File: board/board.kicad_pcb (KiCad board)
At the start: 2 copper layers, 21 x 13 mm, 1 part

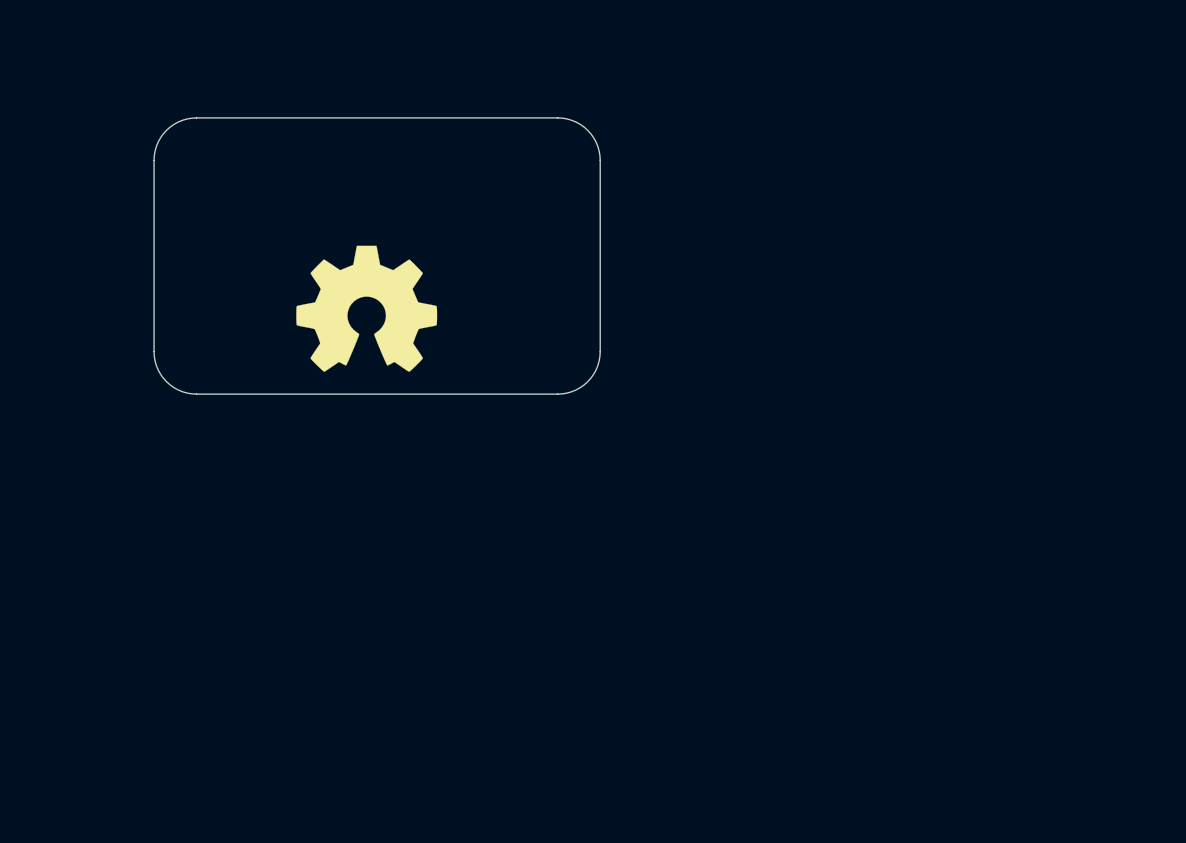
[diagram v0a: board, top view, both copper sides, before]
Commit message: initial
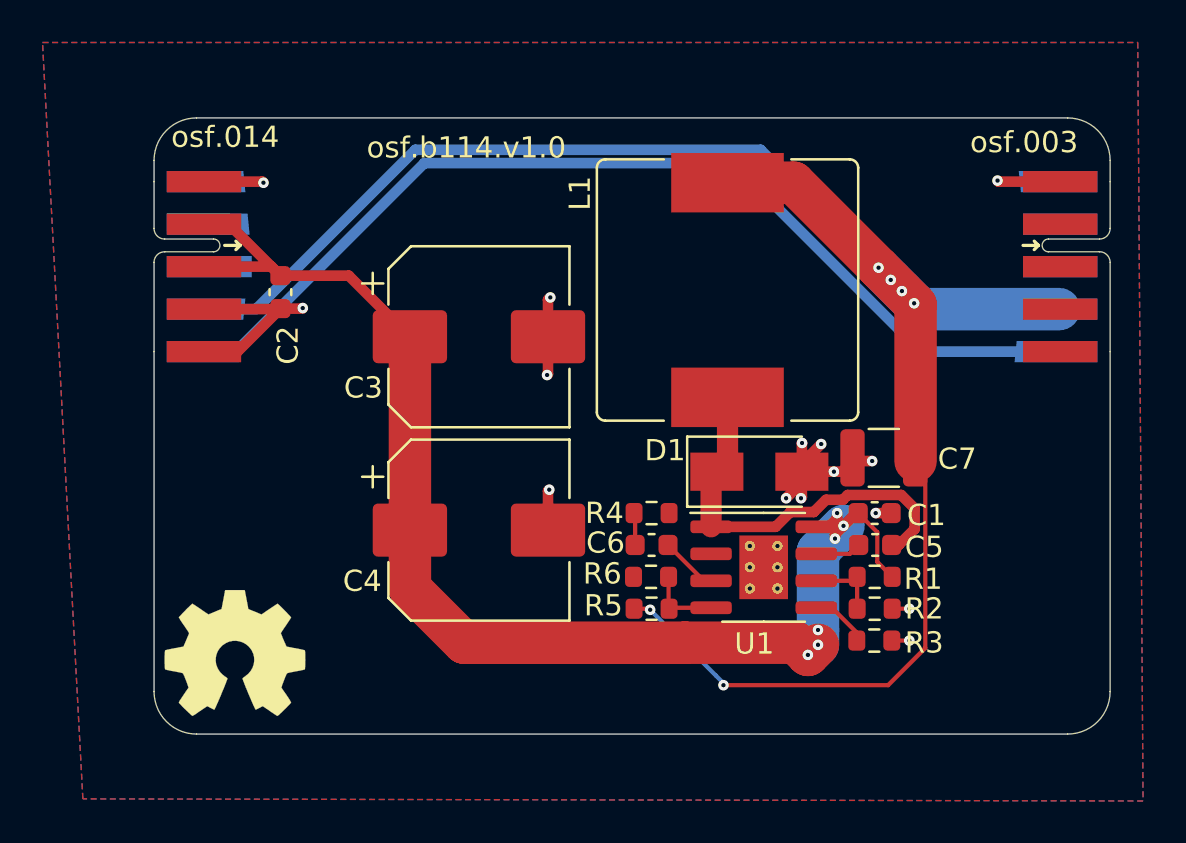
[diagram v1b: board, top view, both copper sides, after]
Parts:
- added C1: 100nF, Capacitor_SMD:C_0603_1608Metric, F.Cu at (173.9, 108.6)
- added C2: 100nF, Capacitor_SMD:C_0603_1608Metric, F.Cu at (145.9, 98.2)
- added C3: 22uF, Capacitor_SMD:CP_Elec_8x10, F.Cu at (155.3, 100.3)
- added C4: 22uF, Capacitor_SMD:CP_Elec_8x10, F.Cu at (155.3, 109.4)
- added C5: 100nF, Capacitor_SMD:C_0603_1608Metric, F.Cu at (173.9, 110.1)
- added C6: 6.8nF, Capacitor_SMD:C_0603_1608Metric, F.Cu at (163.4, 110.1)
- added C7: 100uF, Capacitor_SMD:C_1210_3225Metric, F.Cu at (174.3, 106.0)
- added D1: NRVTSA4100ET3G, Diode_SMD:D_SMA, F.Cu at (168.5, 106.7)
- added J1: 014_PoE_controlled, on_edge:on_edge_2x05_device, F.Cu at (140.0, 97.0)
- added J2: 003_power, on_edge:on_edge_2x05_host, F.Cu at (185.0, 97.0)
- added L1: 33uH, Inductor_SMD:L_Bourns_SRR1210A, F.Cu at (167.0, 98.1)
- added R1: 510k, Resistor_SMD:R_0603_1608Metric, F.Cu at (173.9, 111.6)
- added R2: 100k, Resistor_SMD:R_0603_1608Metric, F.Cu at (173.9, 113.1)
- added R3: 47k, Resistor_SMD:R_0603_1608Metric, F.Cu at (173.9, 114.6)
- added R4: 10k, Resistor_SMD:R_0603_1608Metric, F.Cu at (163.4, 108.6)
- added R5: 2.3k, Resistor_SMD:R_0603_1608Metric, F.Cu at (163.4, 113.1)
- added R6: 1k, Resistor_SMD:R_0603_1608Metric, F.Cu at (163.4, 111.6)
- added U1: BD9G341AEFJ-E2, Package_SO:SOIC-8-1EP_3.9x4.9mm_P1.27mm_EP2.29x3mm_ThermalVias, F.Cu at (168.7, 111.2)
- moved LOGO1 17.3 mm to (143.8, 115.2)
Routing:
- net /step-down/out: track 0.00 -> 90.0 mm, vias 0 -> 6
- net /step-down/in: track 0.00 -> 62.3 mm, vias 0 -> 6
- net Net-(J1-Pad10): track 0.00 -> 47.6 mm
- net GND: track 0.00 -> 32.3 mm, vias 0 -> 15
- net Net-(C5-Pad1): track 0.00 -> 19.2 mm
- net Net-(R5-Pad2): track 0.00 -> 3.50 mm
- net Net-(R1-Pad2): track 0.00 -> 3.50 mm
- net Net-(R3-Pad1): track 0.00 -> 2.77 mm
- net Net-(C6-Pad1): track 0.00 -> 2.72 mm
- net Net-(C5-Pad2): track 0.00 -> 2.17 mm
- net Net-(C6-Pad2): track 0.00 -> 1.52 mm
- added copper zone on B.Cu, net GND
- added copper zone on F.Cu, net GND
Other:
- board size 21 x 13 mm -> 45 x 29 mm
- board text added: "osf.003"
- board text added: "osf.014"
- board text added: "osf.b114.v1.0"
